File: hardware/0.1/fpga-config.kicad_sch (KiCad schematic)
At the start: 31 parts, among them J2 JTAG, J5 USB_C_Receptacle_USB2.0, Q1 BSS138, SW1 SW_Push, U1 ECP5U_12_CABGA256, U4 USBLC6-2SC6, U6 W25Q128JVSIQ

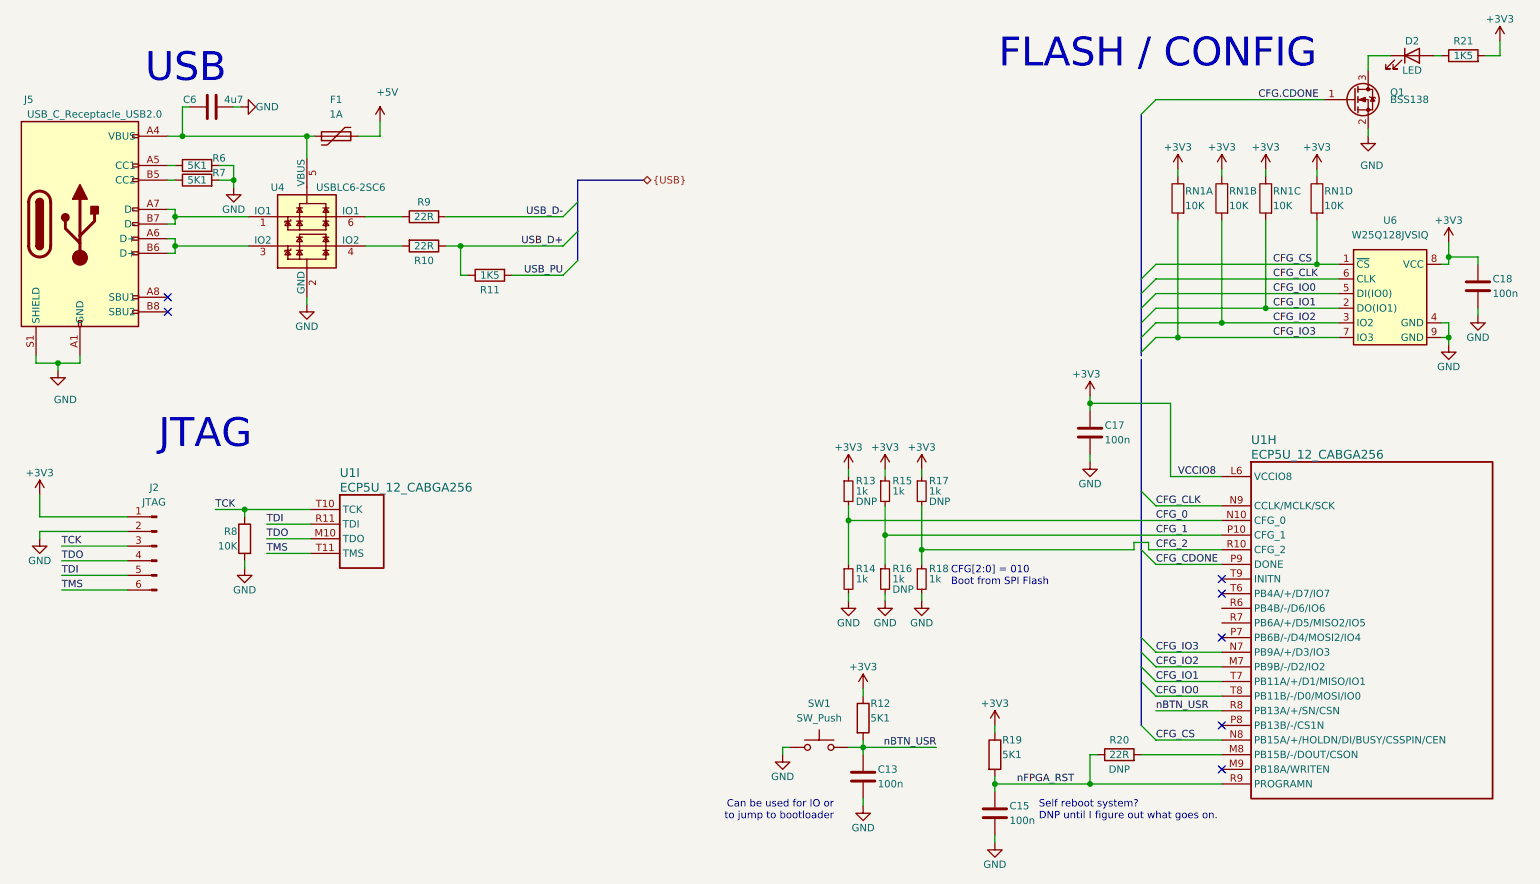
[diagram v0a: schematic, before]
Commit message: half IO routed
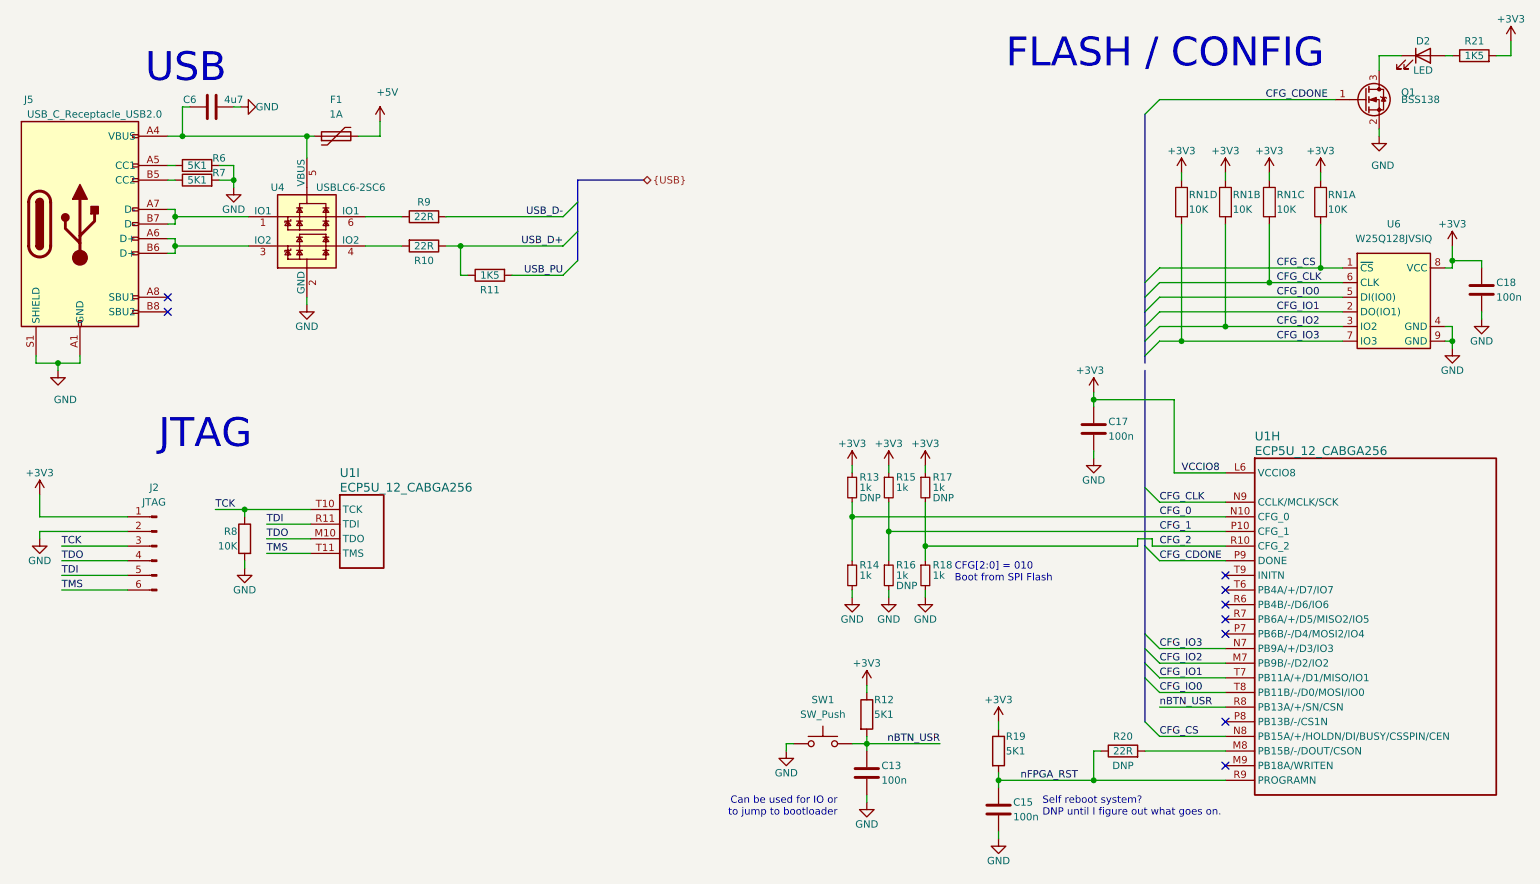
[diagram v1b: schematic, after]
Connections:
- net CFG.CDONE is gone; now on net CFG_CDONE: Q1.1 (G)
- net CFG_CLK: now also RN1.2
- net CFG_CS: now also RN1.4; no longer RN1.1
- net CFG_IO1: no longer RN1.2
- net CFG_IO3: now also RN1.1; no longer RN1.4
- no-connect marks 7 -> 9
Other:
- moved on the sheet: C13, C15, C17, C18, D2, Q1, R12, R13, R14, R15, R16, R17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
